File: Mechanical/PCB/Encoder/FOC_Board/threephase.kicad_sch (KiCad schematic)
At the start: 37 parts, among them J4 U, J5 V, J6 W, Q1 CSD88537ND, Q2 CSD88537ND, Q3 CSD88537ND, U1 DRV8353RSRGZT

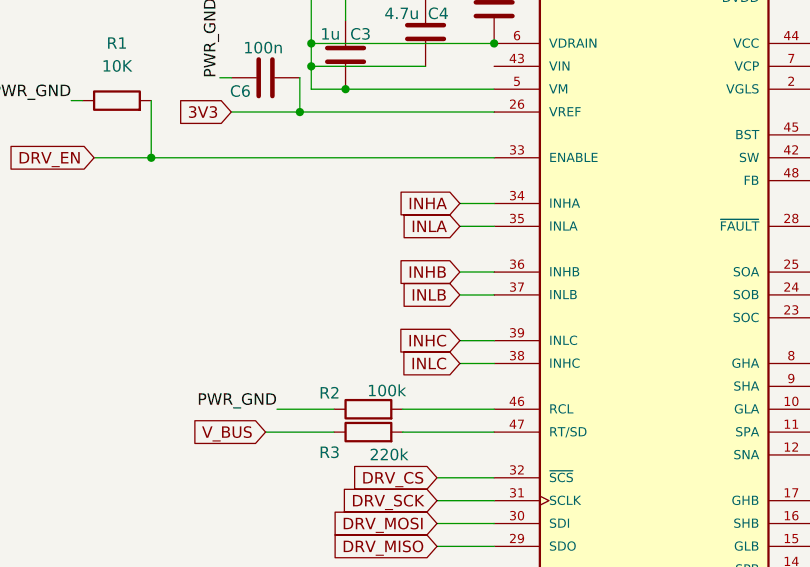
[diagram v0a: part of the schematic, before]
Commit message: layout
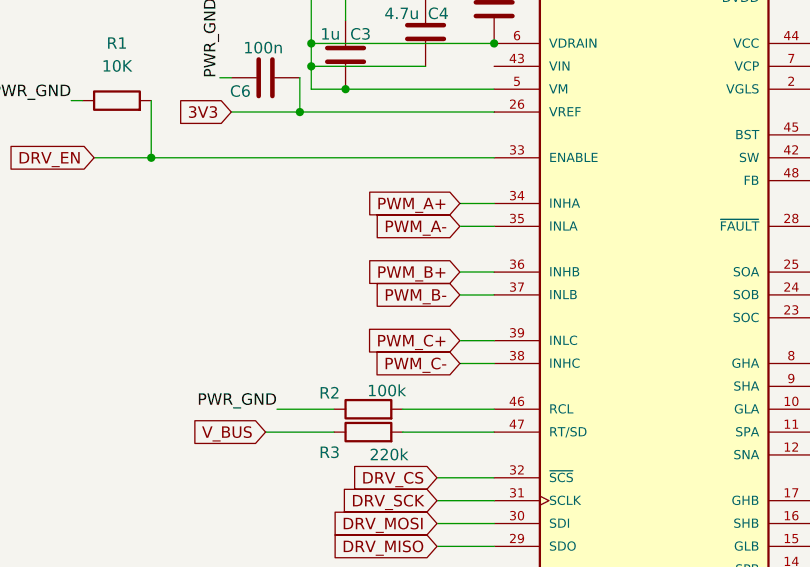
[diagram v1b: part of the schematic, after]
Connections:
- net INHA renamed PWM_A+
- net INHB renamed PWM_B+
- net INHC renamed PWM_C+
- net INLA renamed PWM_A-
- net INLB renamed PWM_B-
- net INLC renamed PWM_C-
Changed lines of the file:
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@@
 		)
 	)
-	(global_label "INHB"
+	(global_label "PWM_B+"
 		(shape input)
 		(at 69.85 57.15 180)
@@
 		)
 		(property "Intersheetrefs" "${INTERSHEET_REFS}"
-			(at 62.329 57.15 0)
+			(at 58.882 57.15 0)
 			(hide yes)
 			(show_name no)
@@
 		)
 	)
-	(global_label "INLA"
+	(global_label "PWM_A-"
 		(shape input)
 		(at 69.85 52.07 180)
@@
 		)
 		(property "Intersheetrefs" "${INTERSHEET_REFS}"
-			(at 62.8128 52.07 0)
+			(at 59.0634 52.07 0)
 			(hide yes)
 			(show_name no)
@@
 		)
 	)
-	(global_label "INLB"
+	(global_label "PWM_B-"
 		(shape input)
 		(at 69.85 59.69 180)
@@
 		)
 		(property "Intersheetrefs" "${INTERSHEET_REFS}"
-			(at 62.6314 59.69 0)
+			(at 58.882 59.69 0)
 			(hide yes)
 			(show_name no)
@@
 		)
 	)
-	(global_label "INHA"
+	(global_label "PWM_A+"
 		(shape input)
 		(at 69.85 49.53 180)
@@
 		)
 		(property "Intersheetrefs" "${INTERSHEET_REFS}"
-			(at 62.5104 49.53 0)
+			(at 59.0634 49.53 0)
 			(hide yes)
 			(show_name no)
@@
 		)
 	)
-	(global_label "INHC"
+	(global_label "PWM_C+"
 		(shape input)
 		(at 69.85 64.77 180)
@@
 		)
 		(property "Intersheetrefs" "${INTERSHEET_REFS}"
-			(at 62.329 64.77 0)
+			(at 58.882 64.77 0)
 			(hide yes)
 			(show_name no)
@@
 		)
 	)
-	(global_label "INLC"
+	(global_label "PWM_C-"
 		(shape input)
 		(at 69.85 67.31 180)
@@
 		)
 		(property "Intersheetrefs" "${INTERSHEET_REFS}"
-			(at 62.6314 67.31 0)
-			(hide yes)
-			(show_name no)
+			(at 58.882 67.31 0)
+			(hide yes)
+			(show_name no)
